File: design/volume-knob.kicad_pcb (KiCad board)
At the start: 2 copper layers, 100 x 100 mm, 32 parts, among them IC1 SGM2212-3.3XKC3G_TR, J1 USB_C_Receptacle, SW1 RotaryEncoder_Switch, SW2 SW_Push, SW3 SW_Push, U1 ESP32-C6-WROOM-1

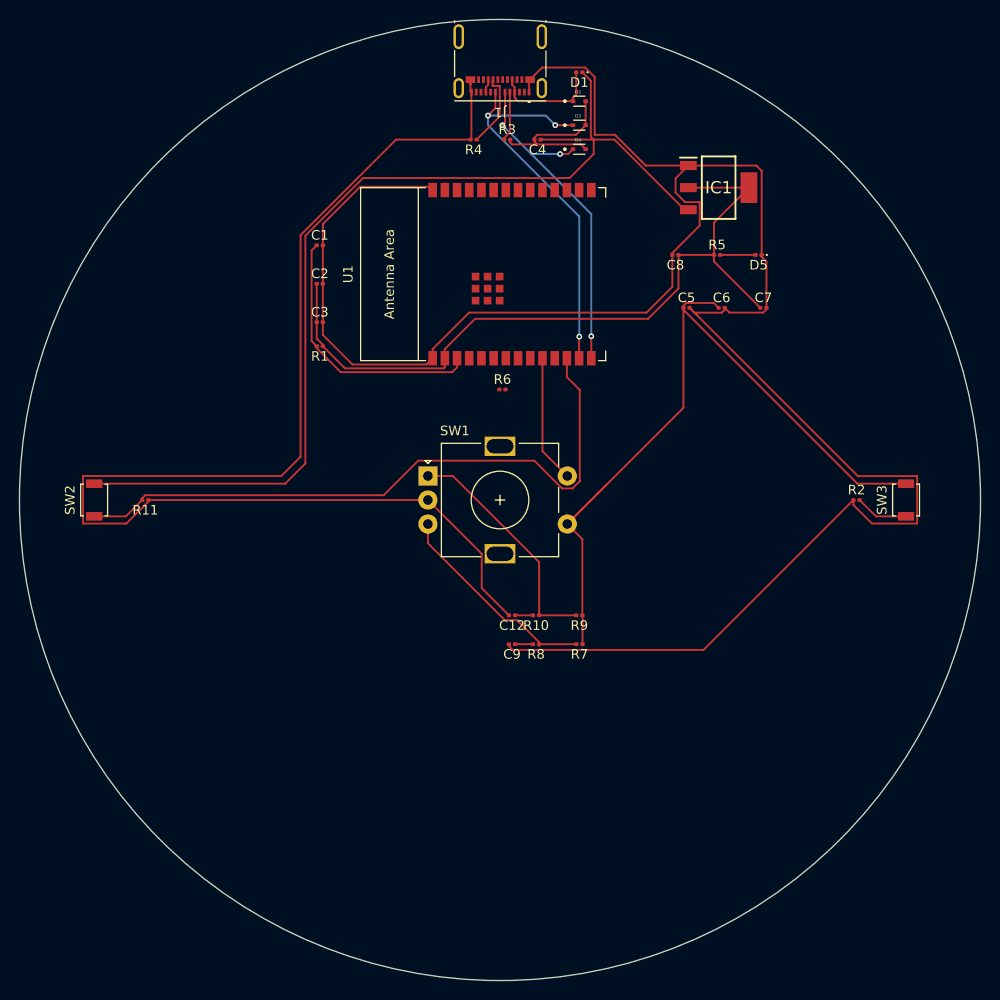
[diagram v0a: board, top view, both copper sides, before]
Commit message: update kicad schematic and pcb
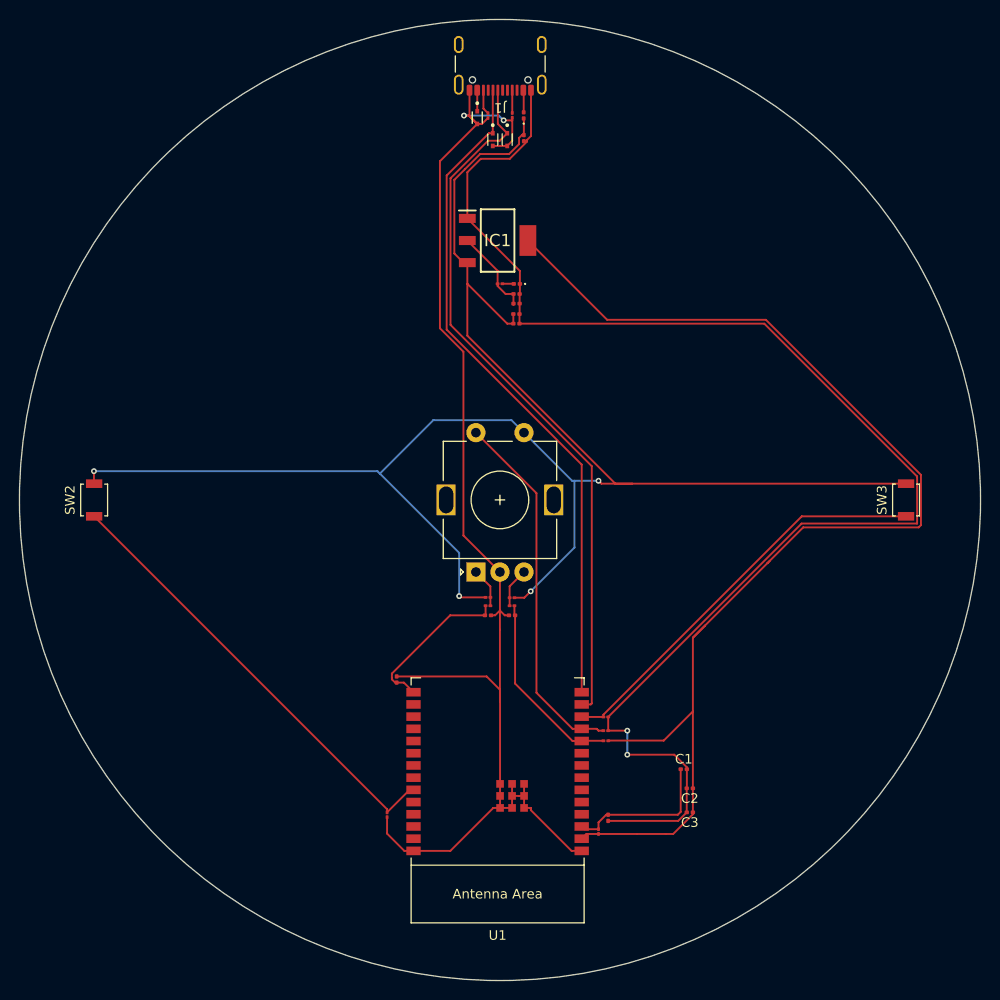
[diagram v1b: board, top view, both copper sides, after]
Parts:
- added C10: 0.1uF, Capacitor_SMD:C_0201_0603Metric, F.Cu at (98.0, 100.2)
- added C11: 0.1uF, Capacitor_SMD:C_0201_0603Metric, F.Cu at (120.0, 114.6)
- added R12: 3.3K, Resistor_SMD:R_01005_0402Metric, F.Cu at (119.8, 106.6)
- J1: footprint Connector_USB:USB_C_Receptacle_Molex_105450-0101 -> Connector_USB:USB_C_Receptacle_GCT_USB4105-xx-A_16P_TopMnt_Horizontal
- R1, R10, R11, R2, R3, R4, R5, R6, R7, R8, R9: footprint Resistor_SMD:R_0201_0603Metric -> Resistor_SMD:R_01005_0402Metric
- moved C1 66.4 mm to (127.9, 109.5)
- moved C2 65.1 mm to (128.5, 111.5), turned to 180 degrees
- moved C3 63.9 mm to (128.5, 114.0), turned to 180 degrees
- moved R1 58.2 mm to (119.0, 116.0), turned to 90 degrees
- moved U1 51.8 mm to (108.5, 109.8), turned to 180 degrees
- moved R11 41.3 mm to (97.0, 114.2), turned to 90 degrees
- moved R6 37.1 mm to (119.8, 105.5)
- moved R2 34.5 mm to (119.8, 104.1), turned to 180 degrees
- moved C7 25.7 mm to (110.5, 60.1)
- moved D5 25.3 mm to (110.5, 59.0)
- moved IC1 23.6 mm to (108.5, 54.5)
- moved R5 22.8 mm to (108.8, 59.0)
- moved C6 21.4 mm to (110.5, 63.2)
- moved C5 17.7 mm to (110.5, 62.2)
- moved C8 17.3 mm to (110.5, 61.1), turned to 0 degrees
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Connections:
- net VBUSB renamed Net-(D1-A)
- C12 pad 1: GPIO10 -> /GPIO9
- C9 pad 1: GPIO9 -> /GPIO8
- D3 pad 1: GPIO12 -> /GPIO12
- D4 pad 1: GPIO13 -> /GPIO13
- J1 pad A6: GPIO13 -> unconnected-(J1-D+-PadA6)
- J1 pad A7: GPIO12 -> /GPIO12
- J1 pad B6: GPIO13 -> /GPIO13
- J1 pad B7: GPIO12 -> unconnected-(J1-D--PadB7)
- R10 pad 2: GPIO10 -> /GPIO9
- R11 pad 2: GPIO11 -> /GPIO15
- R2 pad 2: GPIO15 -> /GPIO11
- R6 pad 1: GPIO8 -> /GPIO10
- R8 pad 2: GPIO9 -> /GPIO8
- SW1 pad S2: GPIO8 -> /GPIO10
- SW2 pad 1: GPIO11 -> /GPIO15
- SW3 pad 1: GPIO15 -> /GPIO11
- U1 pad 10: GPIO8 -> /GPIO8
- U1 pad 11: GPIO10 -> /GPIO10
- U1 pad 12: GPIO11 -> /GPIO11
- U1 pad 13: GPIO12 -> /GPIO12
- U1 pad 14: GPIO13 -> /GPIO13
- U1 pad 15: GPIO9 -> /GPIO9
- U1 pad 23: GPIO15 -> /GPIO15
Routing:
- net GND: track 377.4 -> 289.3 mm, vias 0 -> 4
- net /GPIO12: track 0.00 -> 74.6 mm
- net /GPIO13: track 0.00 -> 70.7 mm
- net GPIO11: track 67.9 -> 0.00 mm
- net VCC_3V3: track 78.8 -> 137.2 mm
- net /GPIO15: track 0.00 -> 47.1 mm
- net /GPIO11: track 0.00 -> 42.5 mm
- net GPIO12: track 41.2 -> 0.00 mm, vias 3 -> 0
- net /GPIO10: track 0.00 -> 38.3 mm
- net GPIO13: track 36.2 -> 0.00 mm, vias 3 -> 0
- net Net-(R10-Pad1): track 24.7 -> 4.15 mm
- net /GPIO8: track 0.00 -> 19.8 mm
- net Net-(R7-Pad2): track 22.1 -> 4.13 mm
- net /GPIO9: track 0.00 -> 16.6 mm
- net GPIO8: track 13.3 -> 0.00 mm
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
